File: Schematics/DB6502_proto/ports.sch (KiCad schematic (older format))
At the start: 20 parts, among them J1 Power plug, J10 System Bus, J2 Controls, J3 AVR ISP, J4 Debug USB, J5 JPR, J6 Debug UART, J7 UART A, J8 UART B, J9 I/O Bus

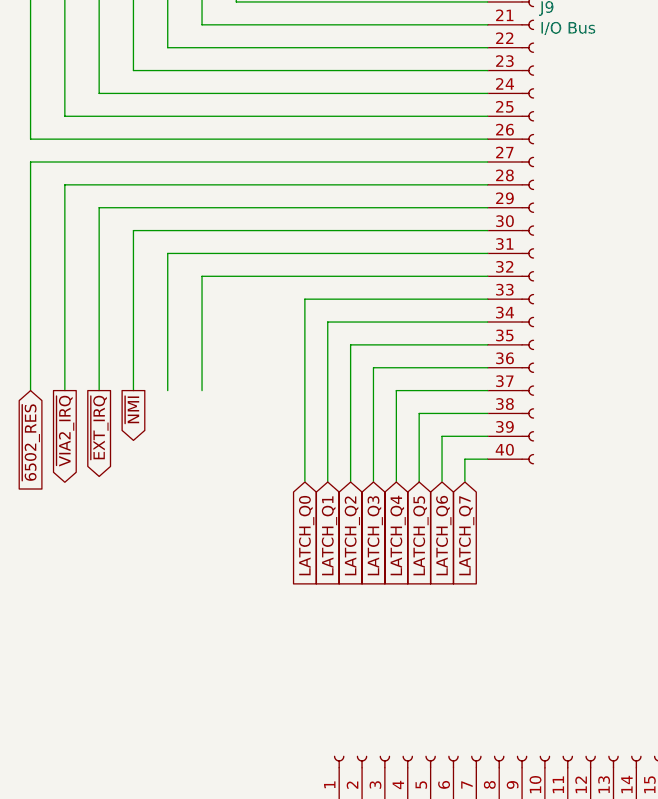
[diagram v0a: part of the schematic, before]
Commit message: Moving things around
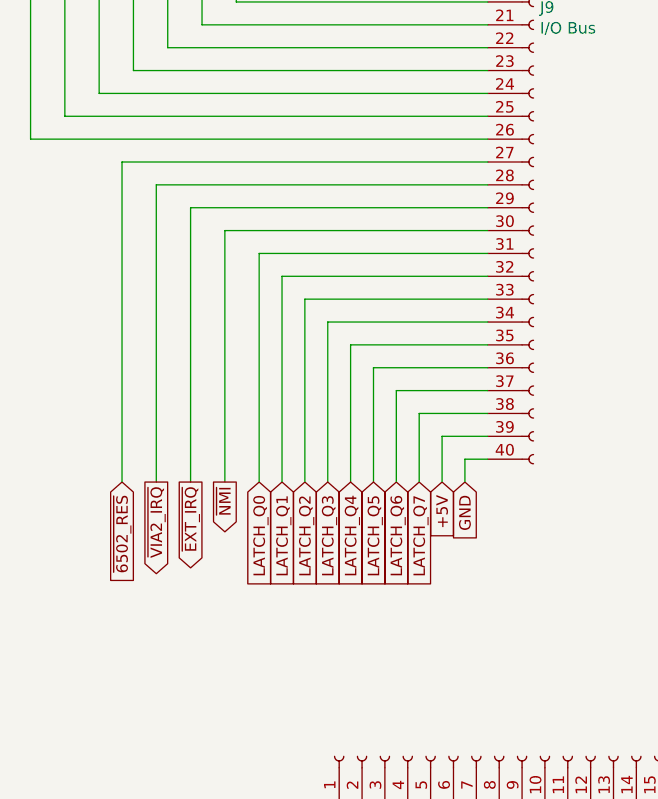
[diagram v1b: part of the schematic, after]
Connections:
- net +5V: now also J9.39 (Pin_39)
- net GND: now also J9.40 (Pin_40)
- net LATCH_Q0: now also J9.31 (Pin_31); no longer J9.33 (Pin_33)
- net LATCH_Q1: now also J9.32 (Pin_32); no longer J9.34 (Pin_34)
- net LATCH_Q2: now also J9.33 (Pin_33); no longer J9.35 (Pin_35)
- net LATCH_Q3: now also J9.34 (Pin_34); no longer J9.36 (Pin_36)
- net LATCH_Q4: now also J9.35 (Pin_35); no longer J9.37 (Pin_37)
- net LATCH_Q5: now also J9.36 (Pin_36); no longer J9.38 (Pin_38)
- net LATCH_Q6: now also J9.37 (Pin_37); no longer J9.39 (Pin_39)
- net LATCH_Q7: now also J9.38 (Pin_38); no longer J9.40 (Pin_40)
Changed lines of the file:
@@
 6502_CLK
 Wire Wire Line
-	1350 4600 1350 3800
-Wire Wire Line
-	1350 3800 3050 3800
+	1750 5000 1750 3800
+Wire Wire Line
+	1750 3800 3050 3800
 Text GLabel 1350 2400 1    50   Input ~ 0
 R~W
 Wire Wire Line
-	1200 4600 1200 3700
-Wire Wire Line
-	1200 3700 3050 3700
-Text GLabel 1050 4600 3    50   Input ~ 0
+	1600 5000 1600 3700
+Wire Wire Line
+	1600 3700 3050 3700
+Text GLabel 1450 5000 3    50   Input ~ 0
 ~6502_RES
 Wire Wire Line
-	1050 4600 1050 3600
-Wire Wire Line
-	1050 3600 3050 3600
+	1450 5000 1450 3600
+Wire Wire Line
+	1450 3600 3050 3600
 Text GLabel 6400 7400 2    50   Input ~ 0
 SYNC
@@
 6502_RDY
 Wire Wire Line
-	1500 4600 1500 3900
-Wire Wire Line
-	1500 3900 3050 3900
-Wire Wire Line
-	1650 4600 1650 4000
-Wire Wire Line
-	1650 4000 3050 4000
-Wire Wire Line
-	1800 4600 1800 4100
-Wire Wire Line
-	1800 4100 3050 4100
+	1900 5000 1900 3900
+Wire Wire Line
+	1900 3900 3050 3900
+Wire Wire Line
+	2050 5000 2050 4000
+Wire Wire Line
+	2050 4000 3050 4000
+Wire Wire Line
+	2150 5000 2150 4100
+Wire Wire Line
+	2150 4100 3050 4100
 $Comp
 L Device:R R2
@@
 Wire Wire Line
 	2950 1000 3050 1000
-Text GLabel 1200 4600 3    50   Output ~ 0
+Text GLabel 1600 5000 3    50   Output ~ 0
 ~VIA2_IRQ
-Text GLabel 1350 4600 3    50   Output ~ 0
+Text GLabel 1750 5000 3    50   Output ~ 0
 ~EXT_IRQ
 Wire Wire Line
@@
 Wire Wire Line
 	5700 4200 6850 4200
-Text GLabel 1500 4600 3    50   Output ~ 0
+Text GLabel 1900 5000 3    50   Output ~ 0
 ~NMI
 Text GLabel 6500 1100 1    50   Input ~ 0
@@
 Wire Wire Line
 	8950 2550 9150 2550
-Text GLabel 2950 5000 3    50   Input ~ 0
+Text GLabel 2750 5000 3    50   Input ~ 0
 LATCH_Q7
-Text GLabel 2850 5000 3    50   Input ~ 0
+Text GLabel 2650 5000 3    50   Input ~ 0
 LATCH_Q6
-Text GLabel 2750 5000 3    50   Input ~ 0
+Text GLabel 2550 5000 3    50   Input ~ 0
 LATCH_Q5
-Text GLabel 2650 5000 3    50   Input ~ 0
+Text GLabel 2450 5000 3    50   Input ~ 0
 LATCH_Q4
-Text GLabel 2550 5000 3    50   Input ~ 0
+Text GLabel 2350 5000 3    50   Input ~ 0
 LATCH_Q3
-Text GLabel 2450 5000 3    50   Input ~ 0
+Text GLabel 2250 5000 3    50   Input ~ 0
 LATCH_Q2
-Text GLabel 2350 5000 3    50   Input ~ 0
+Text GLabel 2150 5000 3    50   Input ~ 0
 LATCH_Q1
-Text GLabel 2250 5000 3    50   Input ~ 0
+Text GLabel 2050 5000 3    50   Input ~ 0
 LATCH_Q0
 Wire Wire Line
@@
 Wire Bus Line
 	2300 6700 3800 6700
+Text GLabel 2850 5000 3    50   Input ~ 0
++5V
+Text GLabel 2950 5000 3    50   Input ~ 0
+GND
 $EndSCHEMATC
